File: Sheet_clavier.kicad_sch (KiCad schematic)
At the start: 15 parts, among them U6 74LS299, U7 74LS299

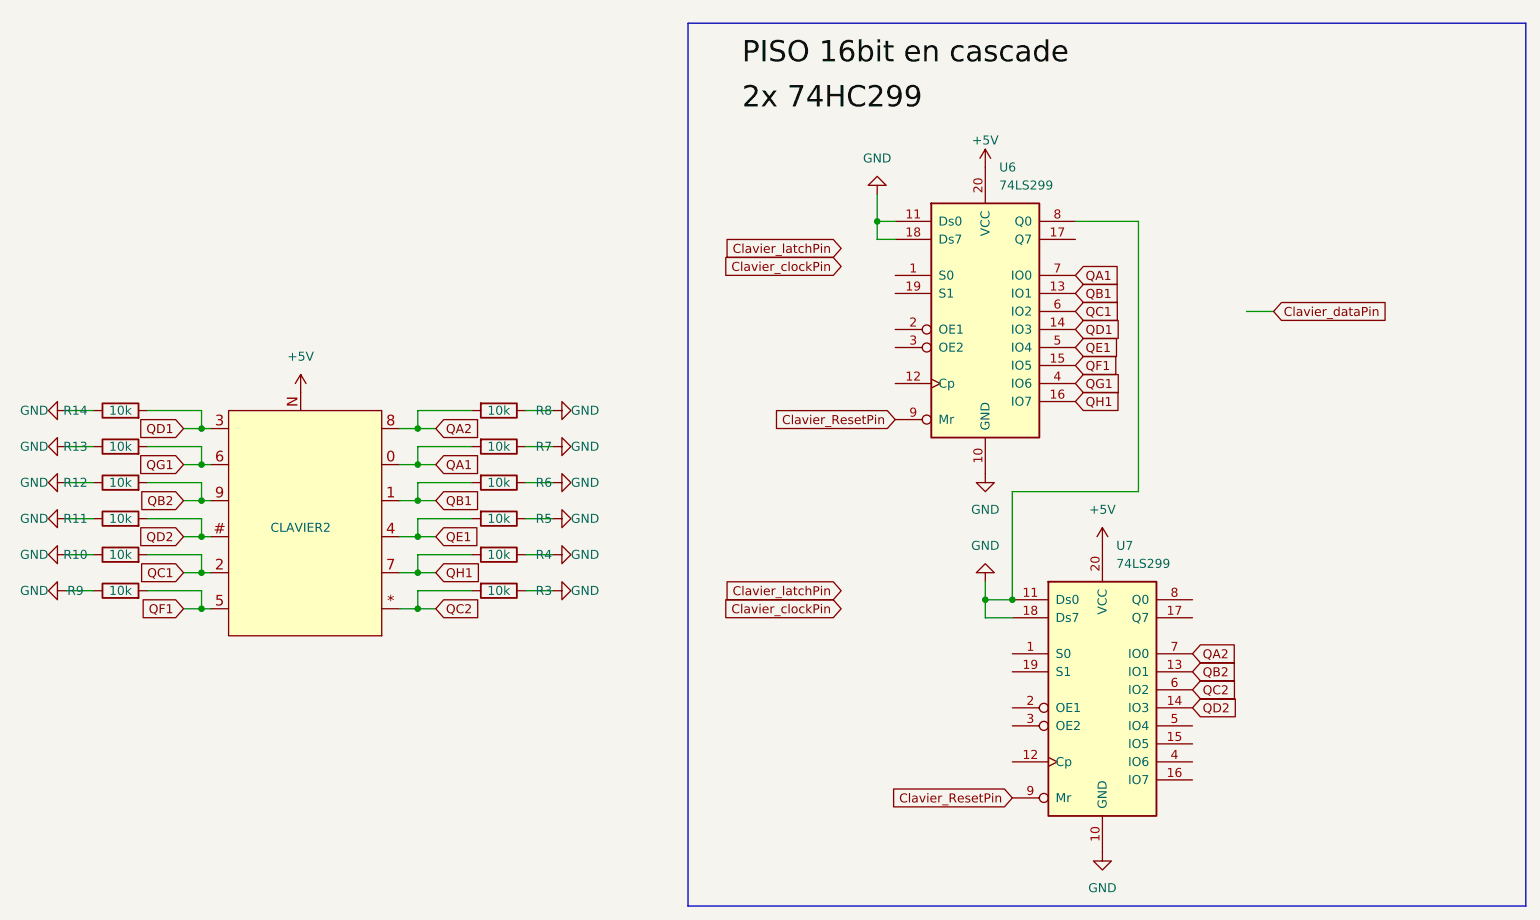
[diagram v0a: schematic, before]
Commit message: clavier re-update with 4021
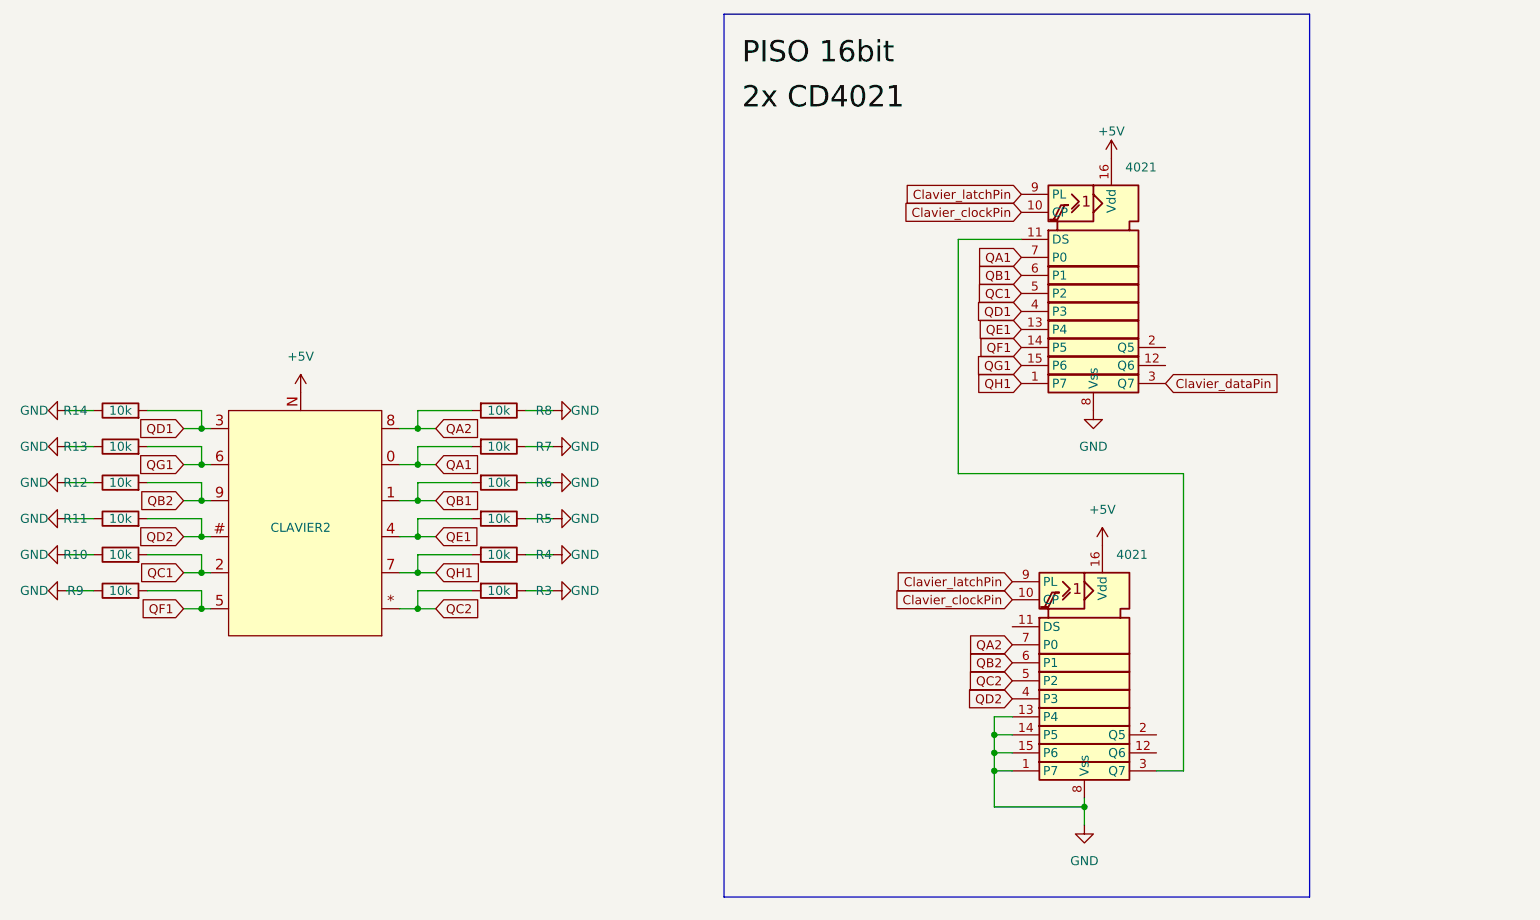
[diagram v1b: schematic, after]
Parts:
- removed U6, U7: 74LS299, symbol 74xx:74LS299
- added U6, U7: 4021, symbol 4xxx_IEEE:4021
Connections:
- net +5V: now also U6.16 (Vdd), U7.16 (Vdd)
- net Clavier_clockPin: now also U6.10 (CP), U7.10 (CP)
- net Clavier_dataPin: now also U6.3 (Q7)
- net Clavier_latchPin: now also U6.9 (PL), U7.9 (PL)
- net GND: now also U6.8 (Vss), U7.1 (P7), U7.13 (P4), U7.14 (P5), U7.15 (P6), U7.8 (Vss)
- net QA1: now also U6.7 (P0)
- net QA2: now also U7.7 (P0)
- net QB1: now also U6.6 (P1)
- net QB2: now also U7.6 (P1)
- net QC1: now also U6.5 (P2)
- net QC2: now also U7.5 (P2)
- net QD1: now also U6.4 (P3)
- net QD2: now also U7.4 (P3)
- net QE1: now also U6.13 (P4)
- net QF1: now also U6.14 (P5)
- net QG1: now also U6.15 (P6)
- net QH1: now also U6.1 (P7)
- new net: U6.11 (DS), U7.3 (Q7)
